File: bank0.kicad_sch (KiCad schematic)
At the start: 16 parts, among them U101 xc7z010clg400, U301 W25Q256FVEI

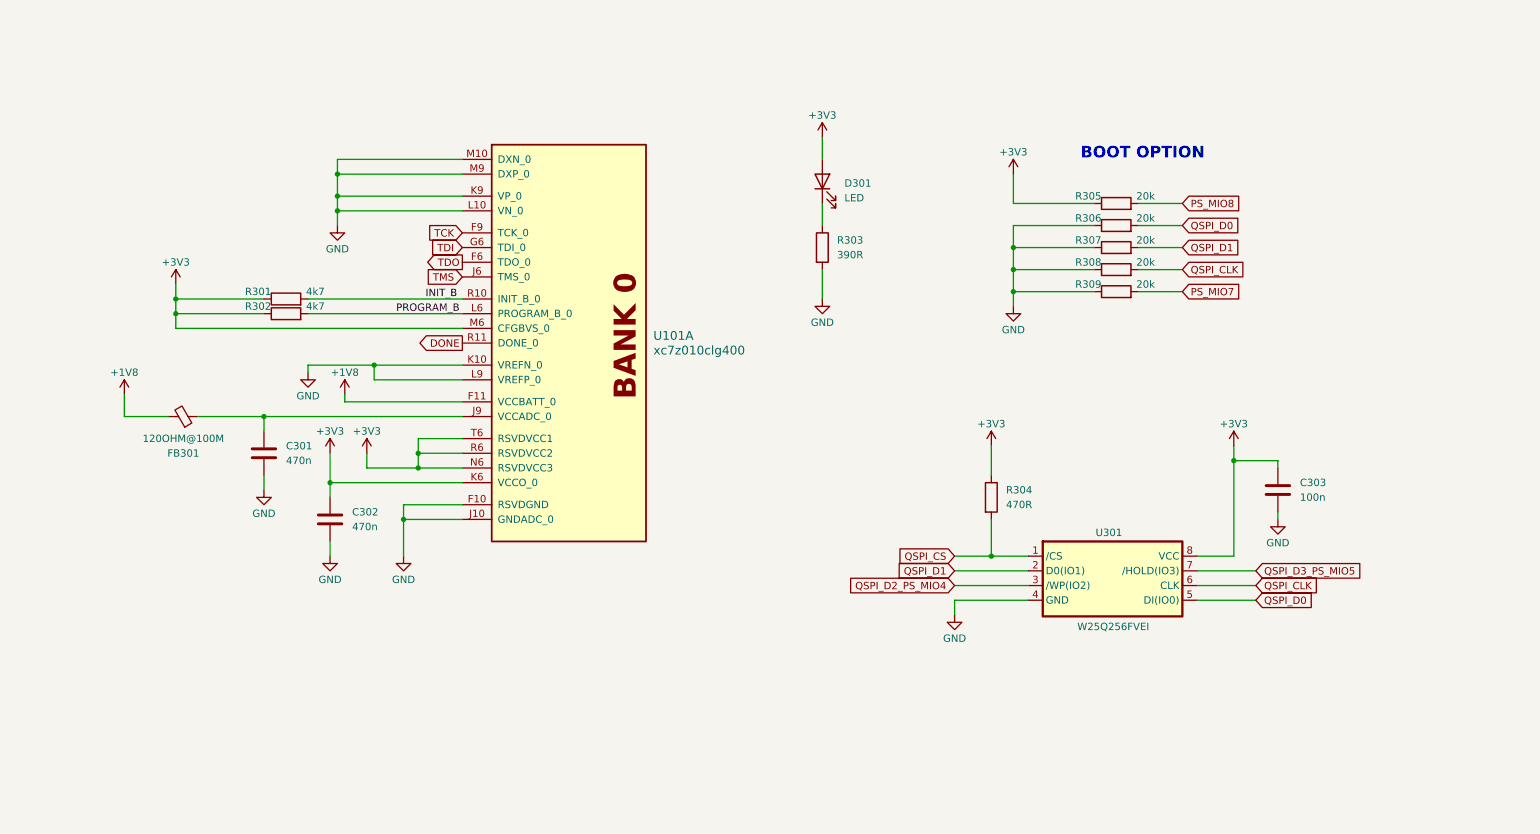
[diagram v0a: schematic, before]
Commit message: feat: continue routing ddr
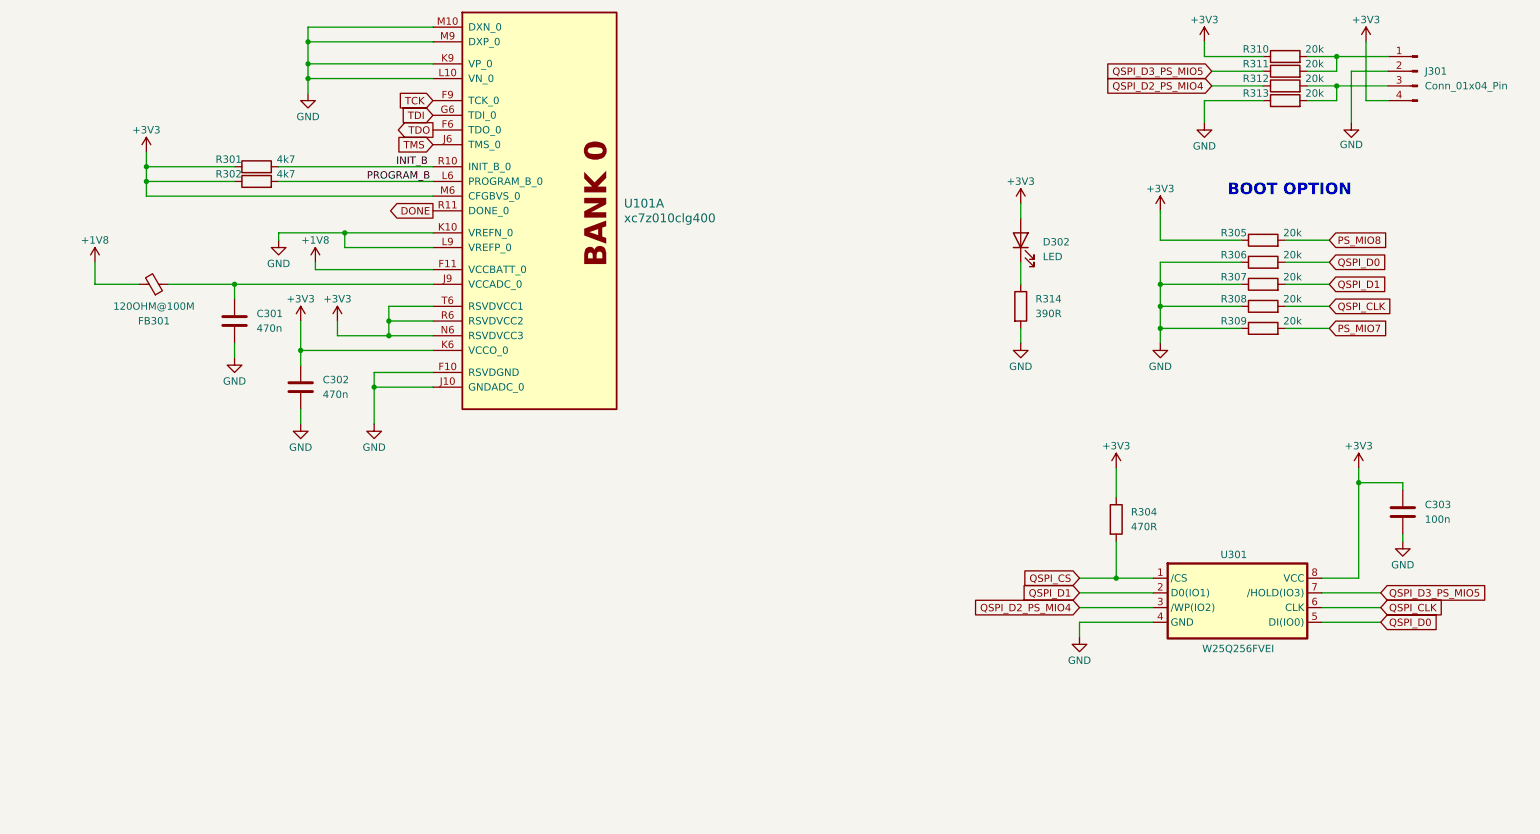
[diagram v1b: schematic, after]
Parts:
- removed D301: LED, symbol Device:LED
- removed R303: 390R, symbol Device:R
- added D302: LED, symbol Device:LED
- added J301: Conn_01x04_Pin, symbol Connector:Conn_01x04_Pin
- added R310, R311, R312, R313: 20k, symbol Device:R
- added R314: 390R, symbol Device:R
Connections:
- net +3V3: now also D302.2 (A), J301.4 (Pin_4), R310.1
- net GND: now also J301.2 (Pin_2), R313.1, R314.2
- net QSPI_D2_PS_MIO4: now also R312.1
- net QSPI_D3_PS_MIO5: now also R311.1
- new net: J301.3 (Pin_3), R312.2, R313.2
- new net: D302.1 (K), R314.1
- new net: J301.1 (Pin_1), R310.2, R311.2
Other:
- moved on the sheet: C301, C302, C303, FB301, R301, R302, R304, R305, R306, R307, R308, R309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

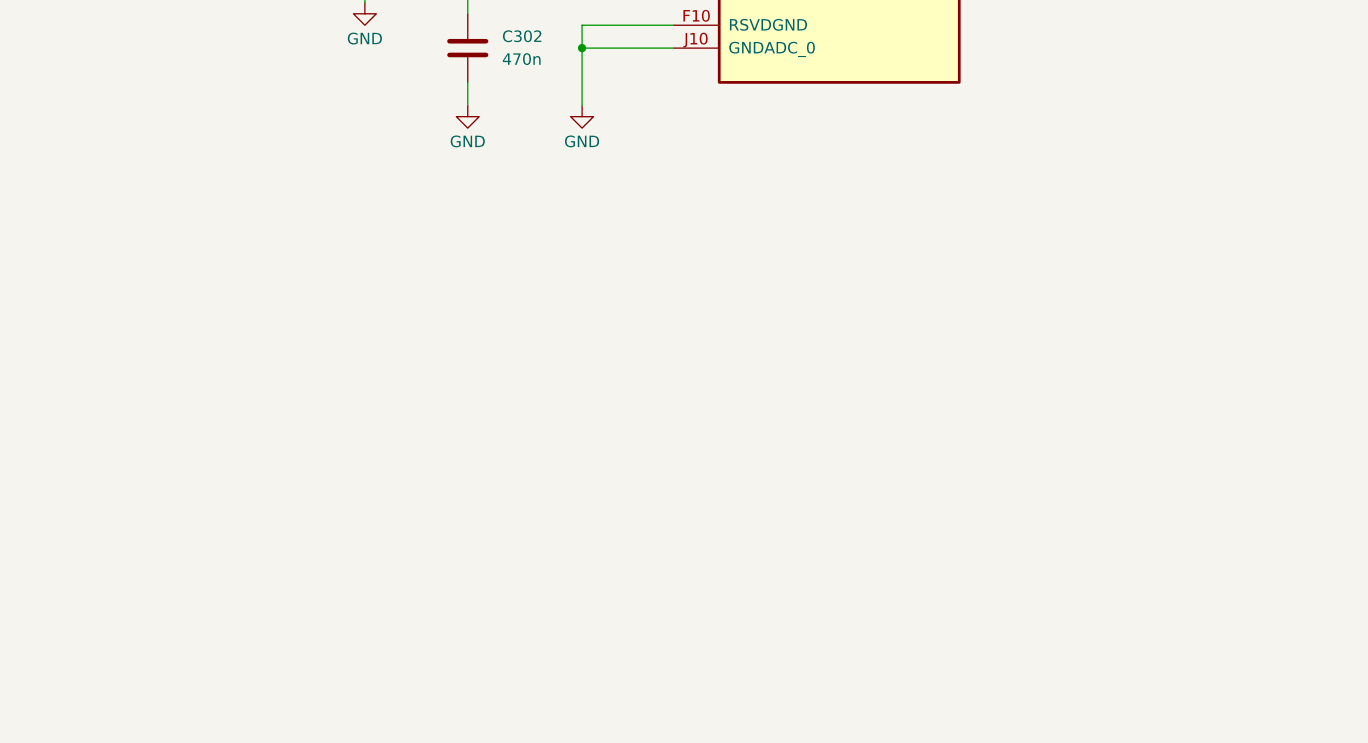
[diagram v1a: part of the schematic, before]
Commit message: feat: continue sch design
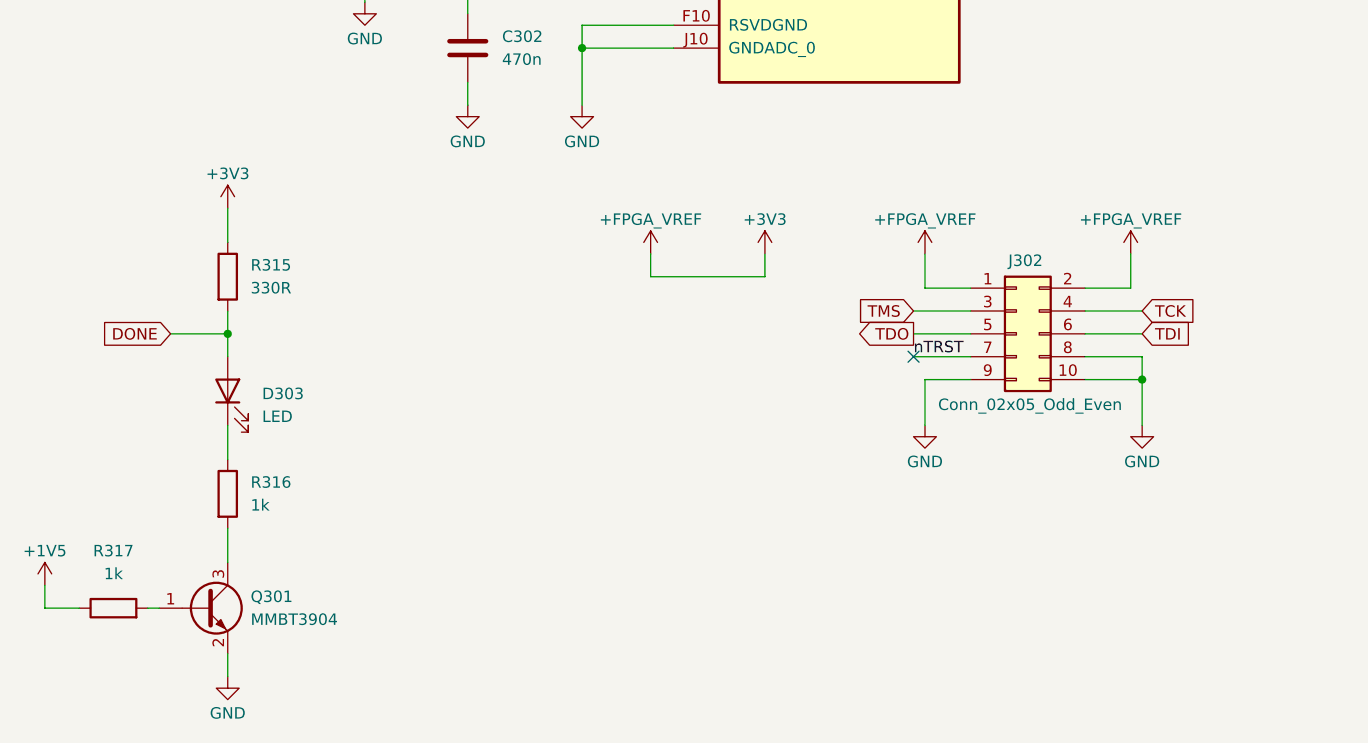
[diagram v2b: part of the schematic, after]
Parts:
- added D303: LED, symbol Device:LED
- added J302: Conn_02x05_Odd_Even, symbol Connector_Generic:Conn_02x05_Odd_Even
- added Q301: MMBT3904, Package_TO_SOT_SMD:SOT-23, symbol Transistor_BJT:MMBT3904
- added R315: 330R, symbol Device:R
- added R316, R317: 1k, symbol Device:R
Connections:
- net +3V3: now also J302.1 (Pin_1), J302.2 (Pin_2), R315.1
- net DONE: now also D303.2 (A), R315.2
- net GND: now also J302.10 (Pin_10), J302.8 (Pin_8), J302.9 (Pin_9), Q301.2 (E)
- net TCK: now also J302.4 (Pin_4)
- net TDI: now also J302.6 (Pin_6)
- net TDO: now also J302.5 (Pin_5)
- net TMS: now also J302.3 (Pin_3)
- new net: D303.1 (K), R316.1
- new net: Q301.3 (C), R316.2
- new net: Q301.1 (B), R317.2
- new net +1V5: R317.1
- new net nTRST: J302.7 (Pin_7)
- no-connect marks 0 -> 1
